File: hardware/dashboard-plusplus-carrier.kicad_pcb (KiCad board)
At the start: 4 copper layers, 95 x 55 mm, 56 parts, among them J1 XT30U-M, J10a ESP32-DEVKIT-A, J10b ESP32-DEVKIT-B, J13 DEBUG, J14 TRIP + EN, J15 SPARE, J16 SPARE N, J17 IGN + COOLANT, J18 SPARE S, J3 TFT-ILI9488, J6 LDR + FUEL, J8 GPS_PADS, J9 HALL, Q1 IRFR9540N, U4 DPP_DCDC_MODULE

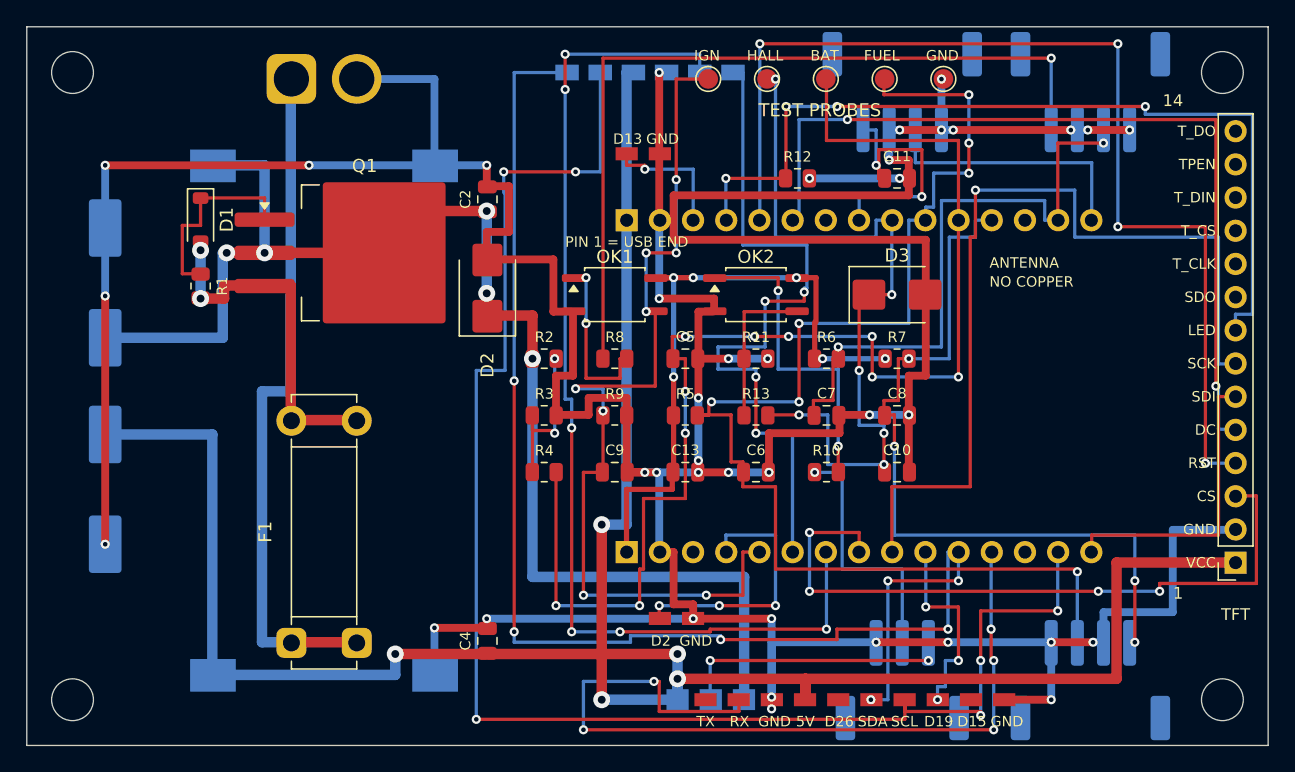
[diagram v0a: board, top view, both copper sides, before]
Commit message: Price wall cuts by leg length, pay debts depth-first: unrouted 3 -> 1
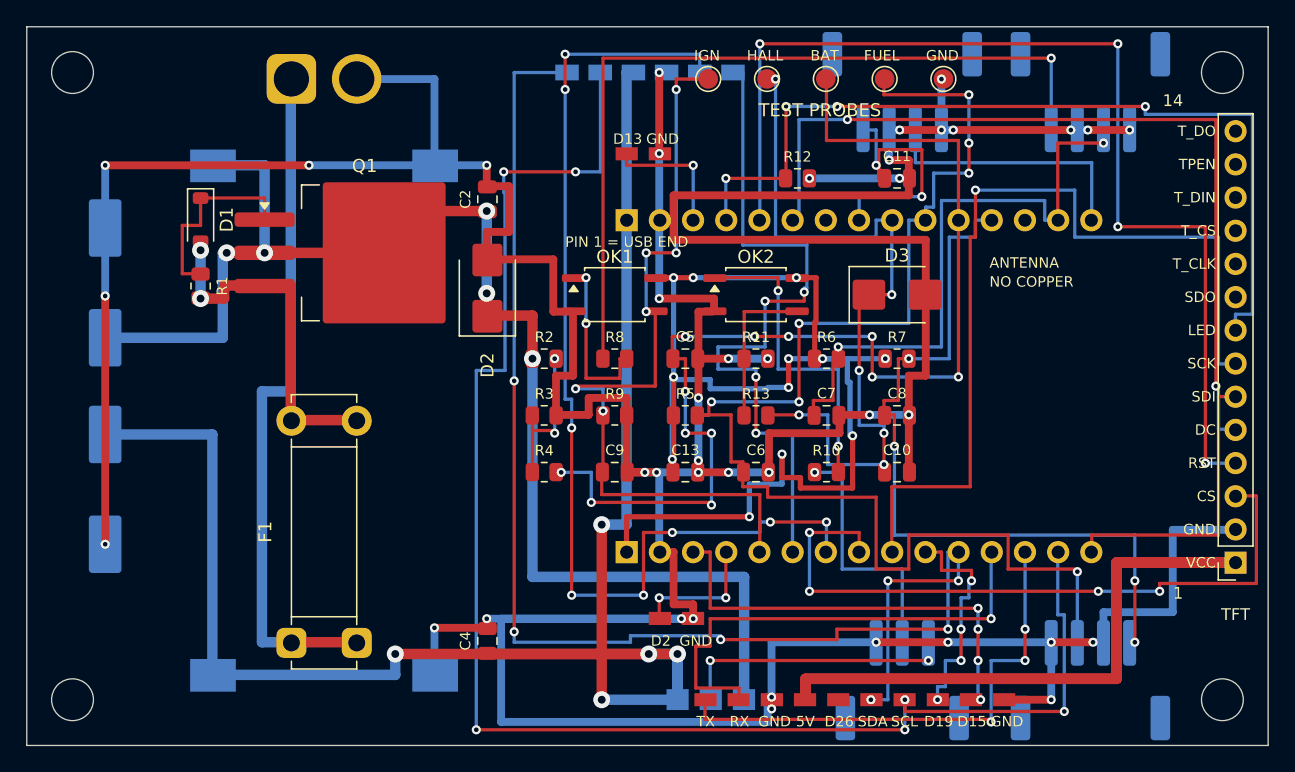
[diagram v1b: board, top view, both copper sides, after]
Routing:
- net V3V3: track 49.0 -> 100.5 mm, vias 6 -> 12
- net V5: track 178.7 -> 227.0 mm
- net DBG_TX: track 0.00 -> 39.0 mm, vias 0 -> 3
- net SPARE_D15: track 0.00 -> 33.9 mm, vias 0 -> 4
- net GND: track 382.7 -> 416.0 mm, vias 39 -> 40
- net DBG_RX: track 63.8 -> 37.0 mm, vias 5 -> 1
- net BAT_SNS: track 99.1 -> 87.7 mm, vias 10 -> 12
- net SPARE_D2: track 20.2 -> 10.0 mm, vias 3 -> 2
- net IGN_SENSE: track 70.7 -> 61.3 mm, vias 8 -> 6
- net FUEL_SNS: track 98.8 -> 104.0 mm
- net SPARE_D22: track 118.4 -> 120.5 mm
- net SPARE_D19: track 15.3 -> 17.3 mm, vias 3 -> 4
- net GPS_TX: track 81.8 -> 80.8 mm, vias 6 -> 8
